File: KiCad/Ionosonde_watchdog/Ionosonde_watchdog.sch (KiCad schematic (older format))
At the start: 42 parts

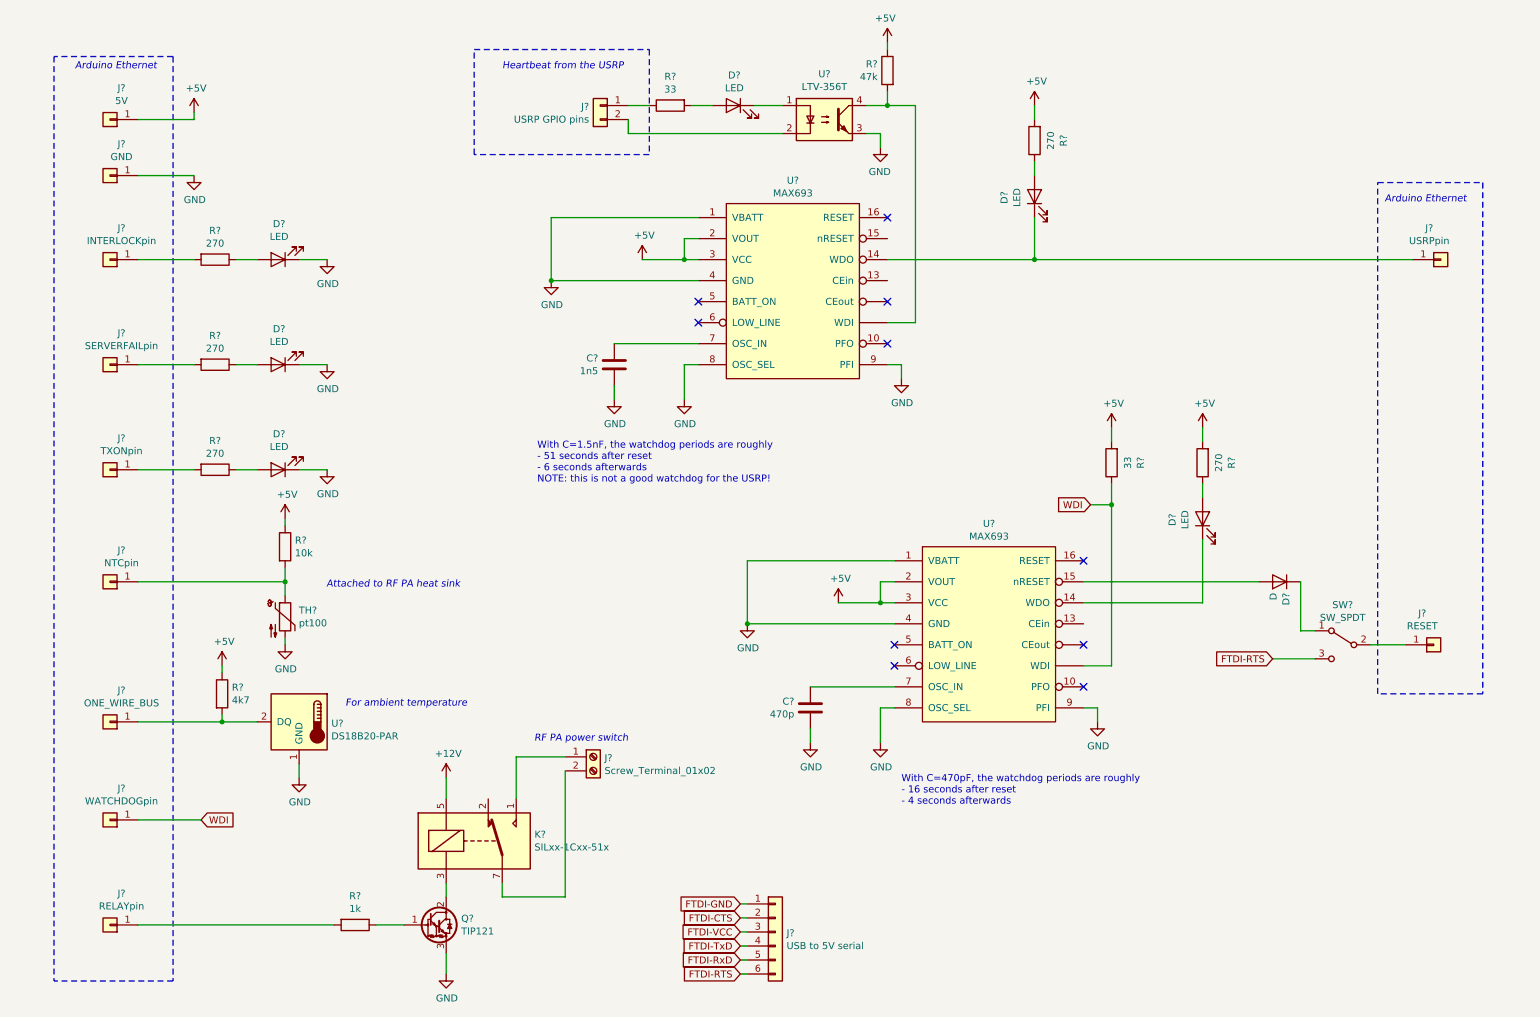
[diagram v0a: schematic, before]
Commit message: New schematics
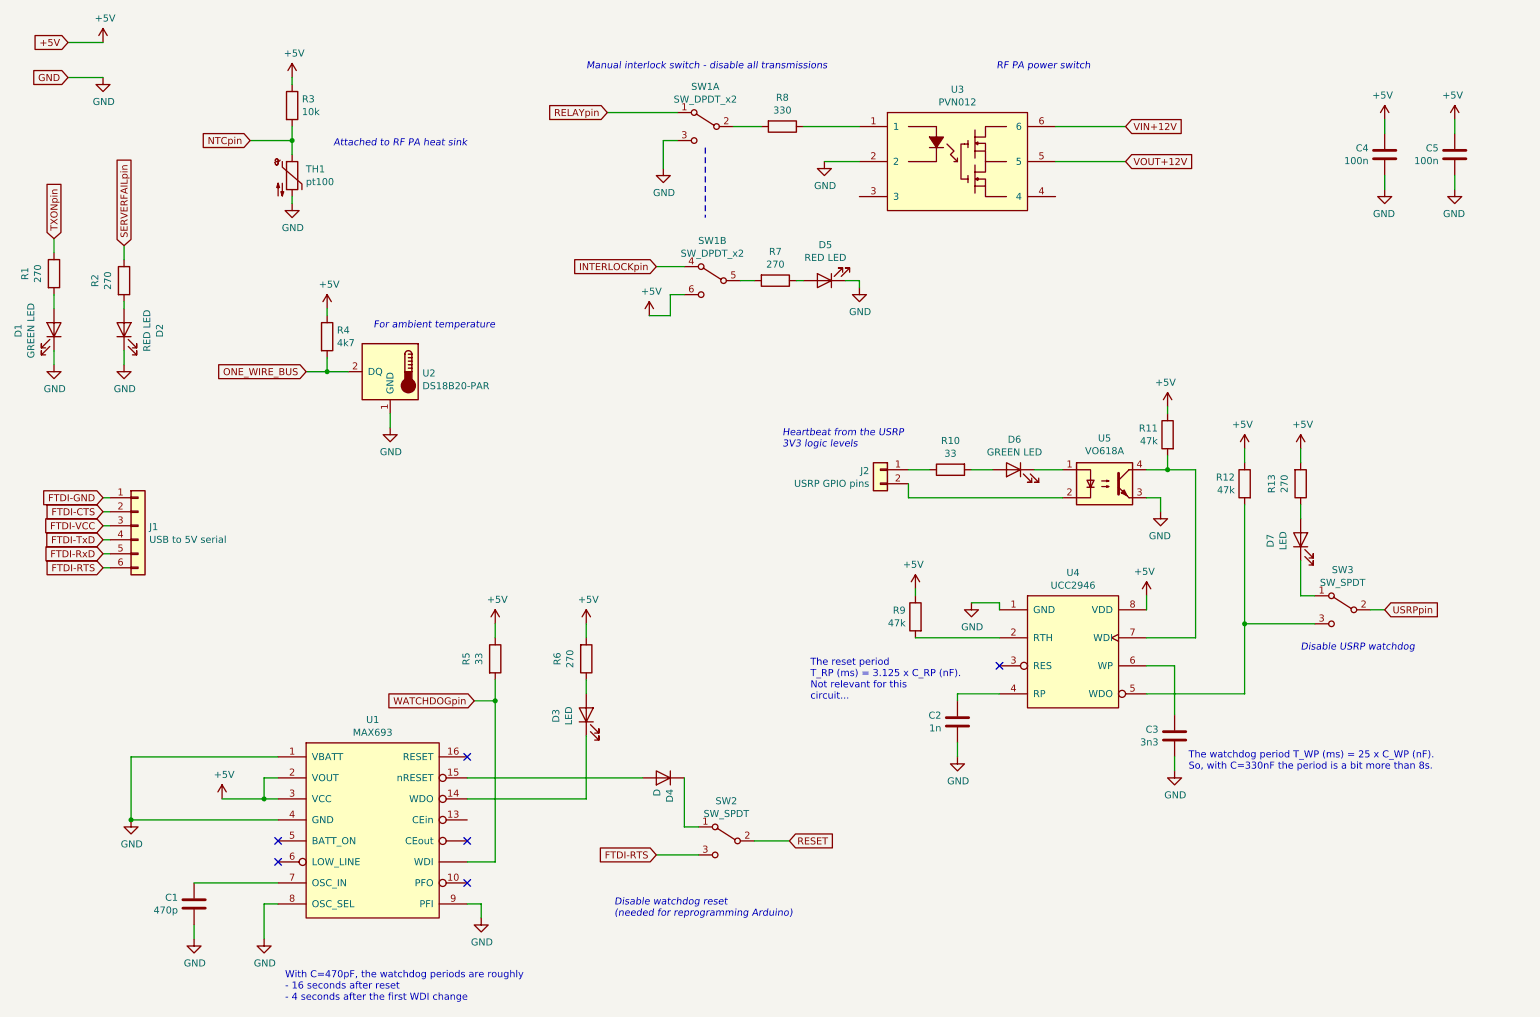
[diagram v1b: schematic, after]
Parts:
- removed D? (x3): LED, symbol Device:LED
- removed J?: INTERLOCKpin, symbol Connector_Generic:Conn_01x01
- removed J?: SERVERFAILpin, symbol Connector_Generic:Conn_01x01
- removed J?: TXONpin, symbol Connector_Generic:Conn_01x01
- removed J?: RELAYpin, symbol Connector_Generic:Conn_01x01
- removed J?: USRPpin, symbol Connector_Generic:Conn_01x01
- removed J?: NTCpin, symbol Connector_Generic:Conn_01x01
- removed J?: ONE_WIRE_BUS, symbol Connector_Generic:Conn_01x01
- removed J?: GND, symbol Connector_Generic:Conn_01x01
- removed J?: 5V, symbol Connector_Generic:Conn_01x01
- removed J?: WATCHDOGpin, symbol Connector_Generic:Conn_01x01
- removed J?: Screw_Terminal_01x02, symbol Connector:Screw_Terminal_01x02
- removed J?: RESET, symbol Connector_Generic:Conn_01x01
- removed K?: SILxx-1Cxx-51x, Relay_THT:Relay_SPDT_StandexMeder_SIL_Form1C, symbol Relay:SILxx-1Cxx-51x
- removed Q?: TIP121, Package_TO_SOT_THT:TO-220-3_Vertical, symbol Transistor_BJT:TIP121
- removed R? (x2): 270, symbol Device:R
- removed U?: MAX693, symbol Ionosonde_watchdog:MAX693
- added C3: 3n3, symbol Device:C
- added C4, C5: 100n, symbol Device:C
- added D1: GREEN LED, symbol Device:LED
- added D2, D5: RED LED, symbol Device:LED
- added R1, R7: 270, symbol Device:R
- added R12, R9: 47k, symbol Device:R
- added SW1: SW_DPDT_x2, symbol Switch:SW_DPDT_x2
- added SW3: SW_SPDT, symbol Switch:SW_SPDT
- added U3: PVN012, symbol pvn012:PVN012
- added U4: UCC2946, symbol ucc2946:UCC2946
- C2: renamed from C?; value 1n5 -> 1n
- D6: renamed from D?; value LED -> GREEN LED
- R8: renamed from R?; value 1k -> 330
- U5: renamed from U?; value LTV-356T -> VO618A
- gave numbers to parts that had none: 18
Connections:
- net +5V: now also R5.1, C4.1, C5.1, R12.1, R9.1, SW1.6 (C), U4.8 (VDD); no longer R5.2
- net GND: now also C3.2, C4.2, C5.2, D1.1 (K), D2.1 (K), D5.1 (K), SW1.3 (C), U3.2, U4.1 (GND)
- net at R8.1: now also U3.1
- net WATCHDOGpin: now reaches U1.~ (WDI)
- net WATCHDOGpin: now also R5.2
- net at R8.2: now also SW1.2 (B)
- net at R2.2: now also D2.2 (A)
- net at D7.1 (K): now also SW3.1 (A)
- net NTCpin: now reaches R3.2, TH1.1
- net ONE_WIRE_BUS: now reaches R4.2, U2.2 (DQ)
- net SERVERFAILpin: now reaches R2.1
- net at R11.2, U5.4: now also U4.7 (WDI)
- net RESET: now reaches SW2.2 (B)
- net at C2.1: now also U4.4 (RP)
- removed net WDI: R5.1, U1.~ (WDI)
- new net: R12.2, SW3.3 (C), U4.5 (WDO)
- new net: R7.2, SW1.5 (B)
- new net: D5.2 (A), R7.1
- new net: R9.2, U4.2 (RTH)
- new net: C3.1, U4.6 (WP)
- new net: D1.2 (A), R1.2
- new net INTERLOCKpin: SW1.4 (A)
- new net RELAYpin: SW1.1 (A)
- new net TXONpin: R1.1
- new net USRPpin: SW3.2 (B)
- new net VIN+12V: U3.6
- new net VOUT+12V: U3.5
- no-connect marks 10 -> 6
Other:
- note added: "Disable USRP watchdog"
- note added: "Disable watchdog reset\n(needed for reprogramming Arduino)"
- note added: "Heartbeat from the USRP\n3V3 logic levels"
- note added: "Manual interlock switch - disable all transmissions"
- note added: "The reset period\nT_RP (ms) = 3.125 x C_RP (nF). \nNot relevant for this\ncircuit..."
- note added: "The watchdog period T_WP (ms) = 25 x C_WP (nF).\nSo, with C=330nF the period is a bit more than 8s."
- note added: "With C=470pF, the watchdog periods are roughly\n- 16 seconds after reset\n- 4 seconds after the first WDI change"
- note removed: "Arduino Ethernet"
- note removed: "Heartbeat from the USRP"
- note removed: "With C=1.5nF, the watchdog periods are roughly\n- 51 seconds after reset\n- 6 seconds afterwards\nNOTE: this is not a good watchdog for the USRP!"
- note removed: "With C=470pF, the watchdog periods are roughly\n- 16 seconds after reset\n- 4 seconds afterwards"
- moved on the sheet: C1, C2, D3, D4, D6, D7, J1, J2, R10, R11, R13, R2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

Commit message: Added voltage monitoring
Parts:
- added D?: GREEN LED, symbol Device:LED
- added R?: 820, symbol Device:R
- added R?: 33k, symbol Device:R
- added R?: 10k, symbol Device:R
- D3: value LED -> RED LED
- R5: value 33 -> 33k
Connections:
- net GND: now also D?.1 (K), R?.2
- net VOUT+12V: now also R?.1, R?.2
- net WDO: now reaches D3.1 (K), U1.14 (WDO)
- net DISABLE_USRP_INTERLOCK: now reaches D7.1 (K), SW3.1 (A)
- net at R12.2, SW3.3 (C): no longer U4.5 (WDO)
- net nRESET: now reaches D4.1 (K), SW2.1 (A)
- net INTERLOCK_ON: now reaches R7.2, SW1.5 (B)
- net TXONpin renamed TOGGLEpin
- new net: D?.2 (A), R?.1
- new net USRP_WDO: U4.5 (WDO)
- new net VMONpin: R?.1, R?.2
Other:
- note added: "Arduino A0"
- note added: "Arduino A1"
- note added: "Connection fail"
- note added: "Interlock alive"
- note added: "Interlock on"
- note added: "Measure the PA power supply voltage"
- note added: "PA power on"
- note added: "USRP alive"
- note added: "USRP watchdog bypass"
- note added: "Watchdog timeout"
- moved on the sheet: C1, C2, C3, C4, C5, D1, D2, D3, D4, D5, D6, D7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
